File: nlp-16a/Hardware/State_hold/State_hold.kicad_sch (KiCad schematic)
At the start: 15 parts, among them J1 Conn_01x08_Male, J2 Conn_01x08_Male, J3 Conn_01x08_Male, J4 Conn_01x08_Male, J5 Conn_01x08_Male, J6 Conn_01x08_Male, J7 Conn_01x08_Male, J8 Conn_01x08_Male, J9 Conn_01x02_Male

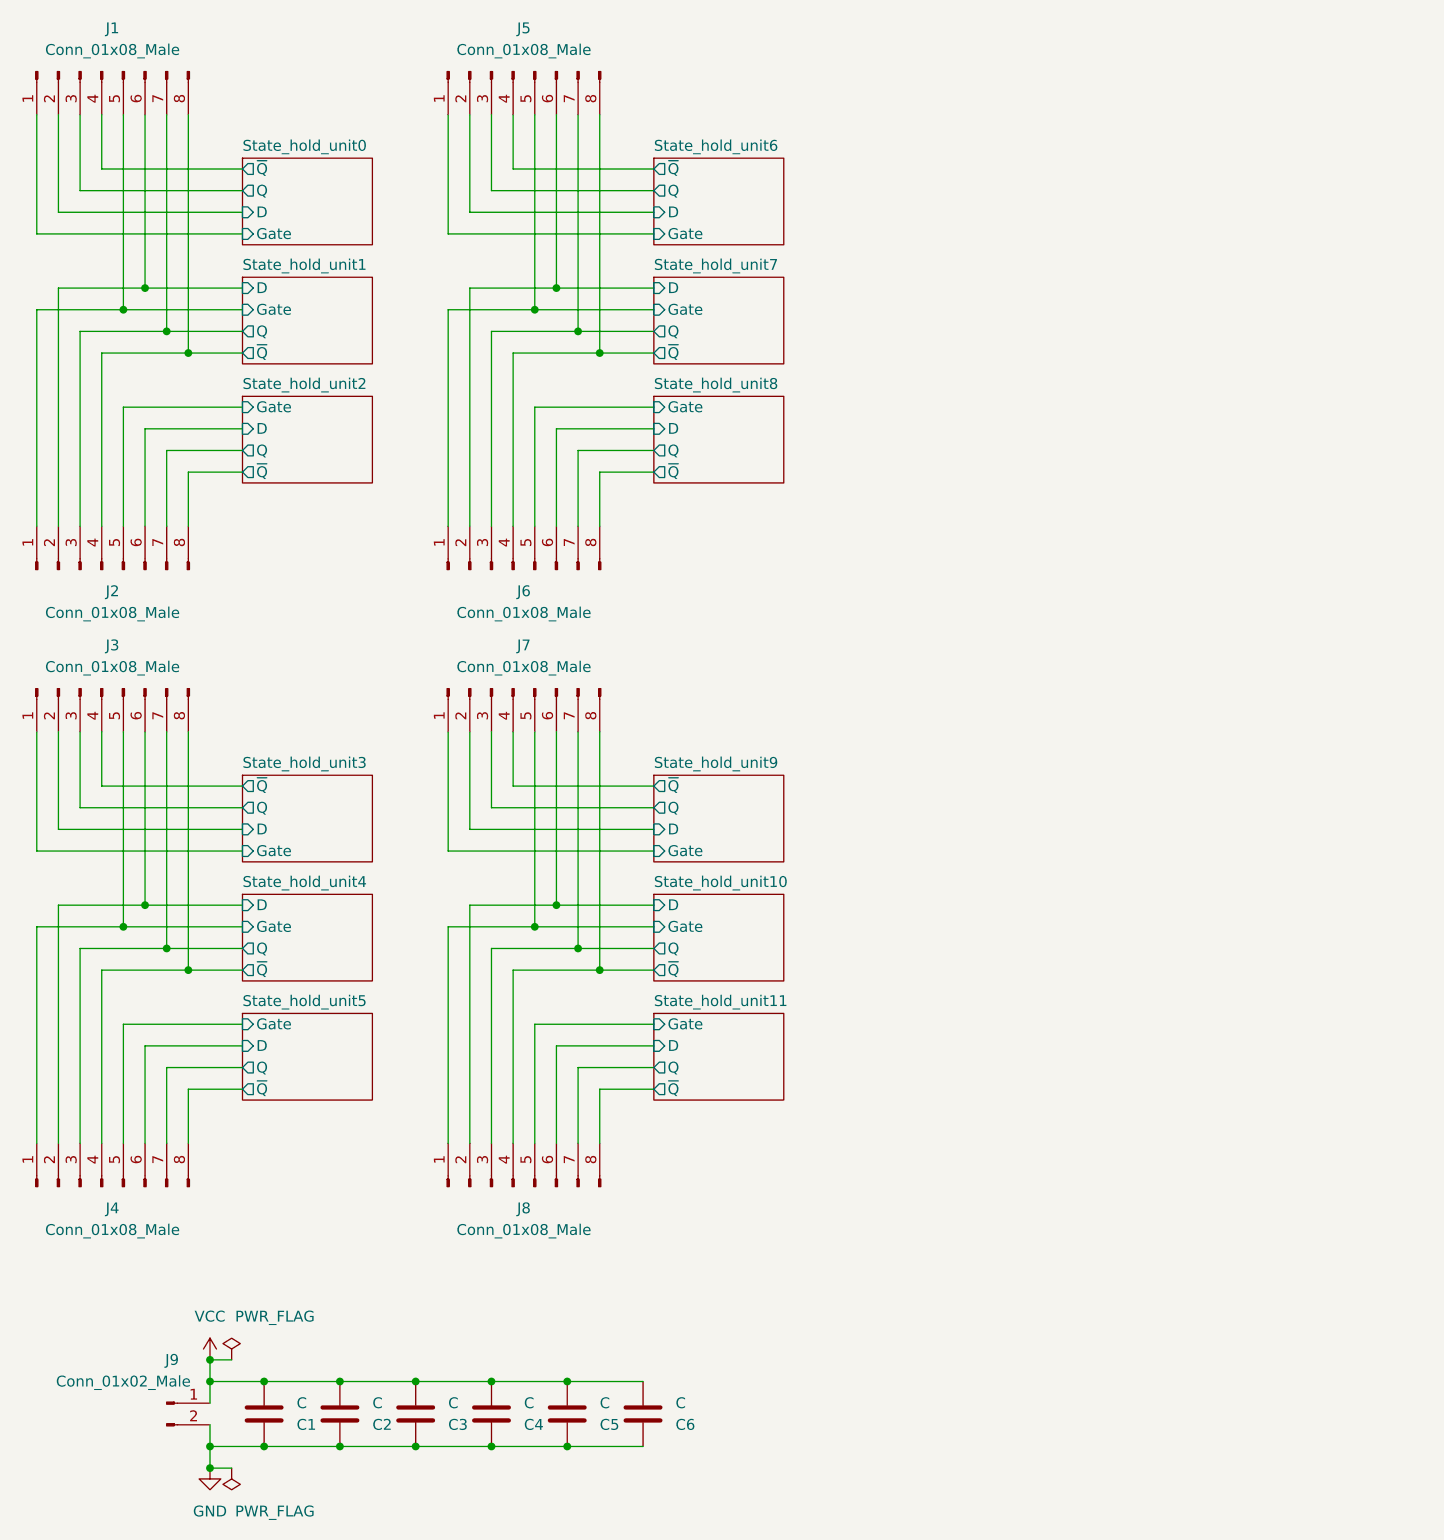
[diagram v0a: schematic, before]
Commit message: ステート保持ラッチ再設計．おそらく問題無し
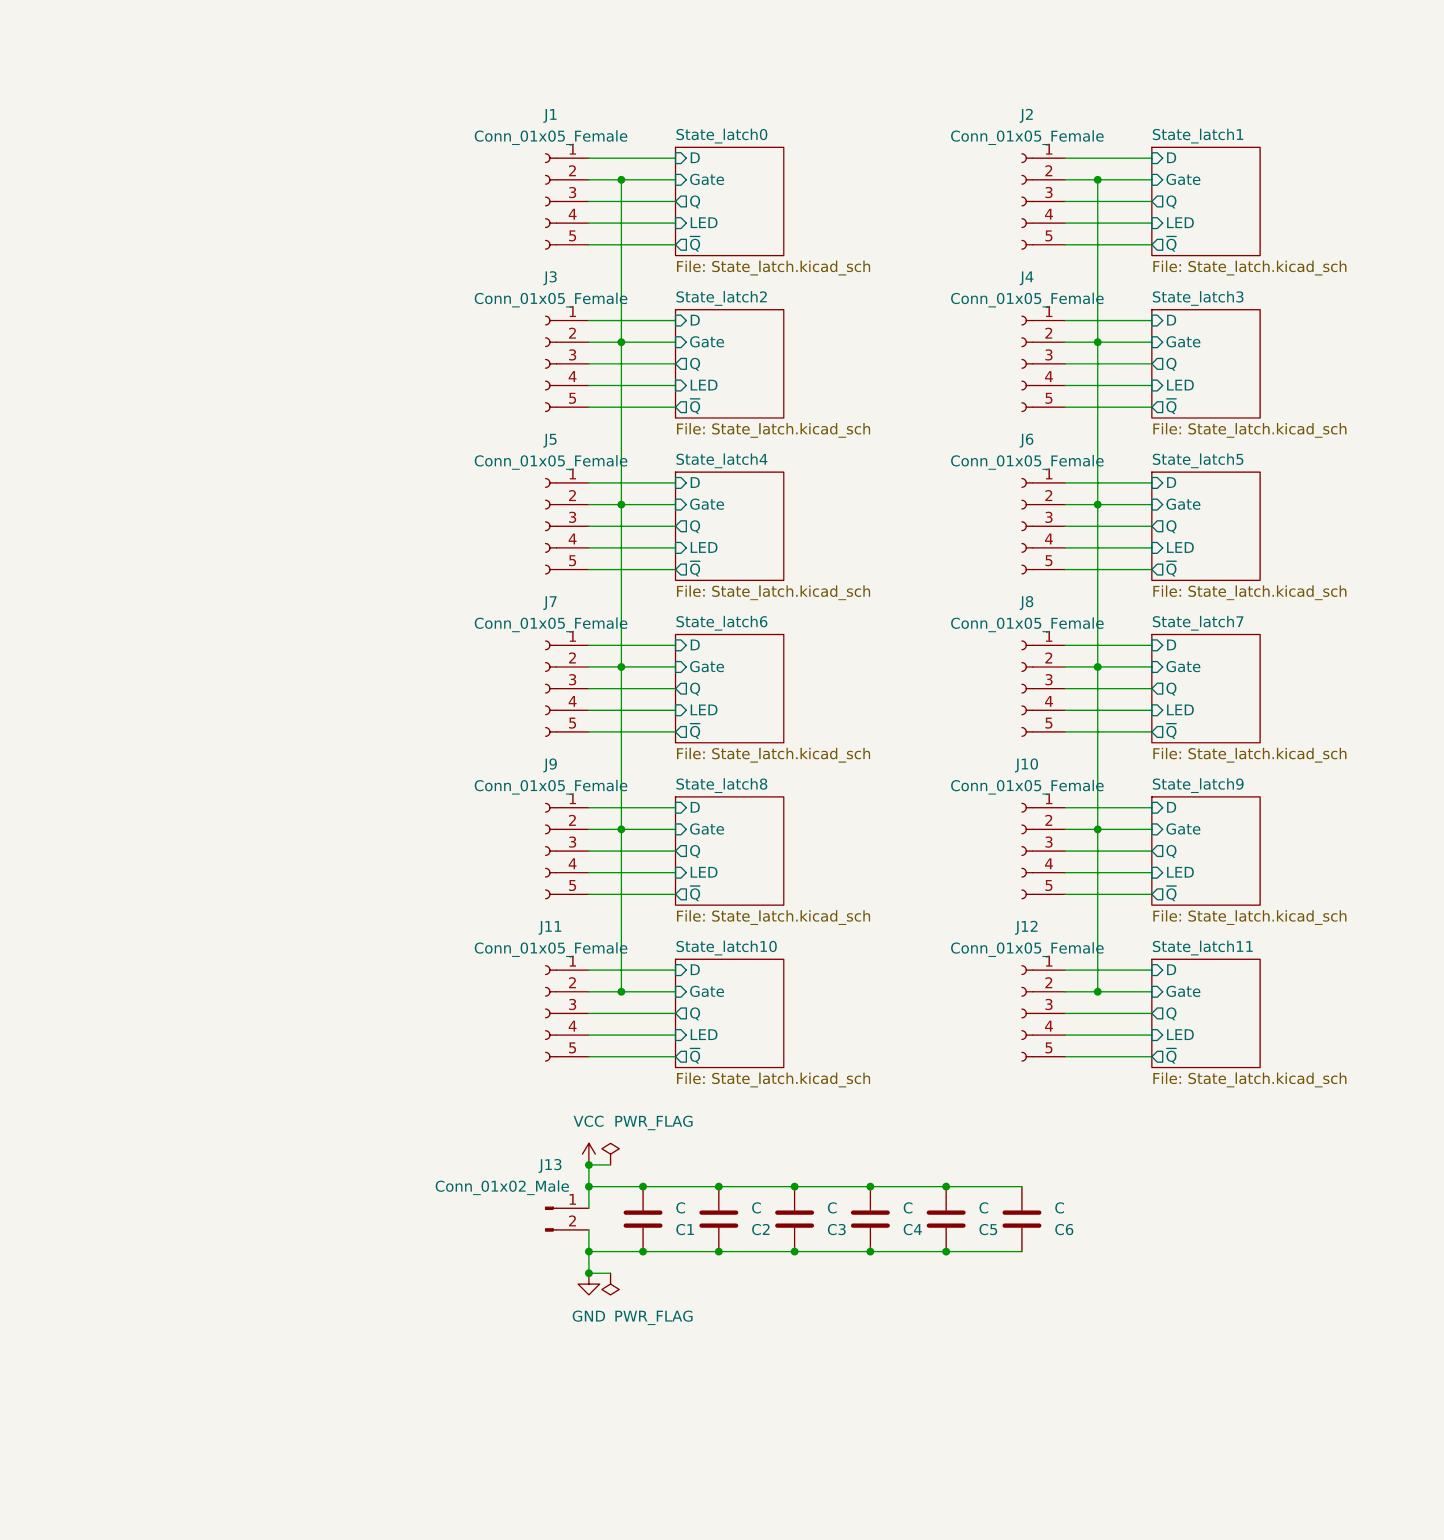
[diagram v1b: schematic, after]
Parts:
- removed J1, J2, J3, J4, J5, J6, J7, J8: Conn_01x08_Male, Connector_PinHeader_2.54mm:PinHeader_1x08_P2.54mm_Vertical, symbol Connector:Conn_01x08_Male
- removed J9: Conn_01x02_Male, Connector_PinHeader_2.54mm:PinHeader_1x02_P2.54mm_Vertical, symbol Connector:Conn_01x02_Male
- added J1, J10, J11, J12, J2, J3, J4, J5, J6, J7, J8, J9: Conn_01x05_Female, Connector_PinSocket_2.54mm:PinSocket_1x05_P2.54mm_Vertical, symbol Connector:Conn_01x05_Female
- added J13: Conn_01x02_Male, Connector_PinHeader_2.54mm:PinHeader_1x02_P2.54mm_Vertical, symbol Connector:Conn_01x02_Male
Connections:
- net GND: now also J13.2 (Pin_2)
- net VCC: now also J13.1 (Pin_1)
- new net State_latch0/D: J1.1 (Pin_1)
- new net State_latch0/Gate: J1.2 (Pin_2), J11.2 (Pin_2), J3.2 (Pin_2), J5.2 (Pin_2), J7.2 (Pin_2), J9.2 (Pin_2)
- new net State_latch0/LED: J1.4 (Pin_4)
- new net State_latch0/Q: J1.3 (Pin_3)
- new net State_latch0/~{Q}: J1.5 (Pin_5)
- new net State_latch1/D: J2.1 (Pin_1)
- new net State_latch1/Gate: J10.2 (Pin_2), J12.2 (Pin_2), J2.2 (Pin_2), J4.2 (Pin_2), J6.2 (Pin_2), J8.2 (Pin_2)
- new net State_latch1/LED: J2.4 (Pin_4)
- new net State_latch1/Q: J2.3 (Pin_3)
- new net State_latch1/~{Q}: J2.5 (Pin_5)
- new net State_latch10/D: J11.1 (Pin_1)
- new net State_latch10/LED: J11.4 (Pin_4)
- new net State_latch10/Q: J11.3 (Pin_3)
- new net State_latch10/~{Q}: J11.5 (Pin_5)
- new net State_latch11/D: J12.1 (Pin_1)
- new net State_latch11/LED: J12.4 (Pin_4)
- new net State_latch11/Q: J12.3 (Pin_3)
- new net State_latch11/~{Q}: J12.5 (Pin_5)
- new net State_latch2/D: J3.1 (Pin_1)
- new net State_latch2/LED: J3.4 (Pin_4)
- new net State_latch2/Q: J3.3 (Pin_3)
- new net State_latch2/~{Q}: J3.5 (Pin_5)
- new net State_latch3/D: J4.1 (Pin_1)
- new net State_latch3/LED: J4.4 (Pin_4)
- new net State_latch3/Q: J4.3 (Pin_3)
- new net State_latch3/~{Q}: J4.5 (Pin_5)
- new net State_latch4/D: J5.1 (Pin_1)
- new net State_latch4/LED: J5.4 (Pin_4)
- new net State_latch4/Q: J5.3 (Pin_3)
- new net State_latch4/~{Q}: J5.5 (Pin_5)
- new net State_latch5/D: J6.1 (Pin_1)
- new net State_latch5/LED: J6.4 (Pin_4)
- new net State_latch5/Q: J6.3 (Pin_3)
- new net State_latch5/~{Q}: J6.5 (Pin_5)
- new net State_latch6/D: J7.1 (Pin_1)
- new net State_latch6/LED: J7.4 (Pin_4)
- new net State_latch6/Q: J7.3 (Pin_3)
- new net State_latch6/~{Q}: J7.5 (Pin_5)
- new net State_latch7/D: J8.1 (Pin_1)
- new net State_latch7/LED: J8.4 (Pin_4)
- new net State_latch7/Q: J8.3 (Pin_3)
- new net State_latch7/~{Q}: J8.5 (Pin_5)
- new net State_latch8/D: J9.1 (Pin_1)
- new net State_latch8/LED: J9.4 (Pin_4)
- new net State_latch8/Q: J9.3 (Pin_3)
- new net State_latch8/~{Q}: J9.5 (Pin_5)
- new net State_latch9/D: J10.1 (Pin_1)
- new net State_latch9/LED: J10.4 (Pin_4)
- new net State_latch9/Q: J10.3 (Pin_3)
- new net State_latch9/~{Q}: J10.5 (Pin_5)
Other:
- removed sheet State_hold_unit0
- removed sheet State_hold_unit1
- removed sheet State_hold_unit10
- removed sheet State_hold_unit11
- removed sheet State_hold_unit2
- removed sheet State_hold_unit3
- removed sheet State_hold_unit4
- removed sheet State_hold_unit5
- removed sheet State_hold_unit6
- removed sheet State_hold_unit7
- removed sheet State_hold_unit8
- removed sheet State_hold_unit9
- added sheet State_latch0 (State_latch.kicad_sch)
- added sheet State_latch1 (State_latch.kicad_sch)
- added sheet State_latch10 (State_latch.kicad_sch)
- added sheet State_latch11 (State_latch.kicad_sch)
- added sheet State_latch2 (State_latch.kicad_sch)
- added sheet State_latch3 (State_latch.kicad_sch)
- added sheet State_latch4 (State_latch.kicad_sch)
- added sheet State_latch5 (State_latch.kicad_sch)
- added sheet State_latch6 (State_latch.kicad_sch)
- added sheet State_latch7 (State_latch.kicad_sch)
- added sheet State_latch8 (State_latch.kicad_sch)
- added sheet State_latch9 (State_latch.kicad_sch)
